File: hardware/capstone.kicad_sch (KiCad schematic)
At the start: 5 parts

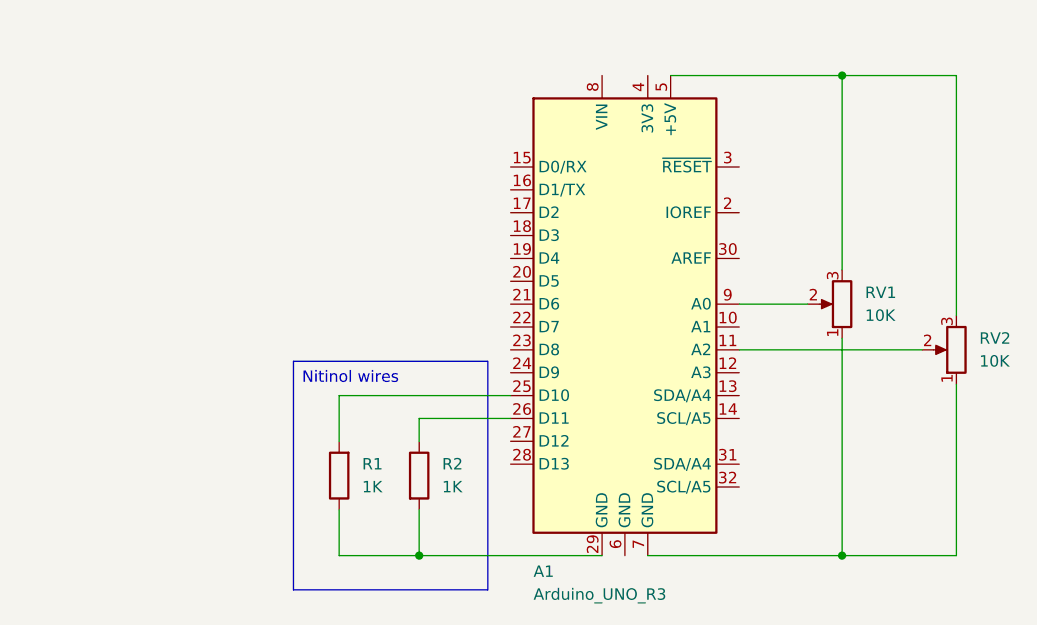
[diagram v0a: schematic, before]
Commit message: add final KiCad project files
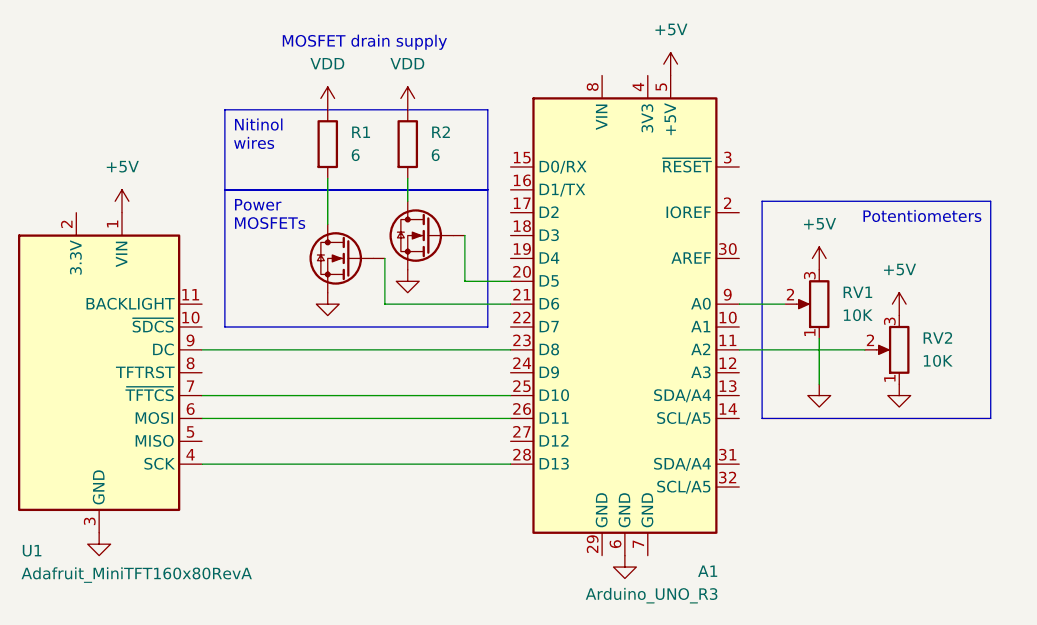
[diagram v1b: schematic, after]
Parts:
- added Q1, Q3: Q_NMOS, symbol Device:Q_NMOS
- added U1: Adafruit_MiniTFT160x80RevA, symbol library:Adafruit_MiniTFT160x80RevA
- R1, R2: value 1K -> 6
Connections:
- net at A1.20 (D5): now also Q3.G
- net at A1.21 (D6): now also Q1.G
- net at A1.23 (D8): now also U1.9 (DC)
- net at R1.2: now also Q1.D; no longer A1.25 (D10)
- net at A1.26 (D11): now also U1.6 (MOSI); no longer R2.1
- net at A1.28 (D13): now also U1.4 (SCK)
- net +5V: now reaches A1.5 (+5V), RV1.3, RV2.3
- net +5V: now also U1.1 (VIN)
- net GND: now reaches A1.6 (GND)
- net GND: now also RV1.1, RV2.1, Q1.S, Q3.S, U1.3 (GND)
- new net: Q3.D, R2.2
- new net: A1.25 (D10), U1.7 (~{TFTCS})
- new net VDD: R1.1, R2.1
- now unconnected: A1.29 (GND), A1.7 (GND)
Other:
- note added: "MOSFET drain supply"
- moved on the sheet: RV1, RV2
